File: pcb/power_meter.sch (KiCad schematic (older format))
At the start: 46 parts, among them J1 USB_B, J2 AudioJack3, J3 Conn_Coaxial, U1 LD1117S33TR_SOT223, U2 ATmega32U4-MU, U3 nRF24L01P, U4 RFX2401C, Y1 16 MHz, Y2 16 MHz

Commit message: separate schematic in multiple sheets; annotate components; power section
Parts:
- removed C? (x2): 22 pF, symbol Device:C
- removed C?: 10 nF, symbol Device:C
- removed C?: 1 nF, symbol Device:C
- removed C?: 33 nF, symbol Device:C
- removed C? (x5): 1.5 pF, symbol Device:C
- removed C?: 0.3 pF, symbol Device:C
- removed C?: 220 pF, symbol Device:C
- removed C?: 1 uF, symbol Device:C
- removed C?: 1 pF, symbol Device:C
- removed C?: 2.2 nF, symbol Device:C
- removed C?: 4.7 nF, symbol Device:C
- removed J3: Conn_Coaxial, symbol Connector:Conn_Coaxial
- removed L? (x2): 2.4 nH, symbol Device:L
- removed L?: 8.2 nH, symbol Device:L
- removed L?: 3.9 nH, symbol Device:L
- removed L?: 2.7 nH, symbol Device:L
- removed R?: 1M, symbol Device:R
- removed R?: 22k, symbol Device:R
- removed R? (x2): 1k, symbol Device:R
- removed R?: 20k, symbol Device:R
- removed U3: nRF24L01P, Package_DFN_QFN:QFN-20-1EP_4x4mm_P0.5mm_EP2.5x2.5mm, symbol RF:nRF24L01P
- removed U4: RFX2401C, QFN50P300X300X60-17N, symbol power_meter-rescue:RFX2401C-RFX2401C
- removed Y2: 16 MHz, symbol Device:Crystal
- added C1, C4: 1 uF, symbol Device:C
- added C2, C3: 10 uF, symbol Device:C
- added C5: 100 nF, symbol Device:C
- added D1: D, symbol Device:D
- added F1: Polyfuse, symbol Device:Polyfuse
- added LOGO1: Logo_Open_Hardware_Small, Symbol:OSHW-Logo2_9.8x8mm_SilkScreen, symbol Graphic:Logo_Open_Hardware_Small
- C10, C7, C8, C9: renamed from C?; footprint (none) -> Capacitor_SMD:C_0402_1005Metric
- J1: footprint (none) -> Connector_USB:USB_B_Lumberg_2411_02_Horizontal
- J2: footprint (none) -> Connector_Audio:Jack_3.5mm_CUI_SJ-3523-SMT_Horizontal
- R5: renamed from R?; footprint (none) -> Resistor_SMD:R_0402_1005Metric
- gave numbers to parts that had none: 4
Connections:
- net GND: now also U1.1 (GND), C1.2, C2.2, C3.2, C4.2, C5.2
- net VBUS: now also U2.14 (VCC), U2.24 (AVCC), U2.34 (VCC), U2.44 (AVCC), C1.1, F1.2
- net VCC: no longer U2.24 (AVCC), U2.44 (AVCC)
- net VDD: now also U1.2 (VO), C3.1, C4.1, C5.1
- net at U1.3 (VI): now also C2.1, D1.1 (K)
- net NRF_SCK renamed SCK
- new net: D1.2 (A), F1.1
- no-connect marks 23 -> 22
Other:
- note added: "Power"
- note added: "Shield is grounded at the\nhost side.\n22 Ohm resistors are\nrequired by the USB standard.\nUSB standard mandatas input\ncapacitance <= 10 uF."
- note added: "USB Connector & Decoupling"
- note removed: "Antenna Matching Network"
- note removed: "Conversion to Unbalanced & Impedance Matching Network"
- note removed: "Decoupling & Support Circuitry"
- note removed: "Nordic Semiconductors nRF24L01P"
- note removed: "RFAxis RFX2401C"
- note removed: "SMA Connector"
- note removed: "Shield is grounded at the\nhost side.\n22 Ohm resistors are\nrequired by the USB standard."
- note removed: "TODO: LINK TO ORIGINAL SCHEMATIC"
- note removed: "USB Connector"
- moved on the sheet: C6, D2, J1, J2, R1, R2, R3, R4, U1

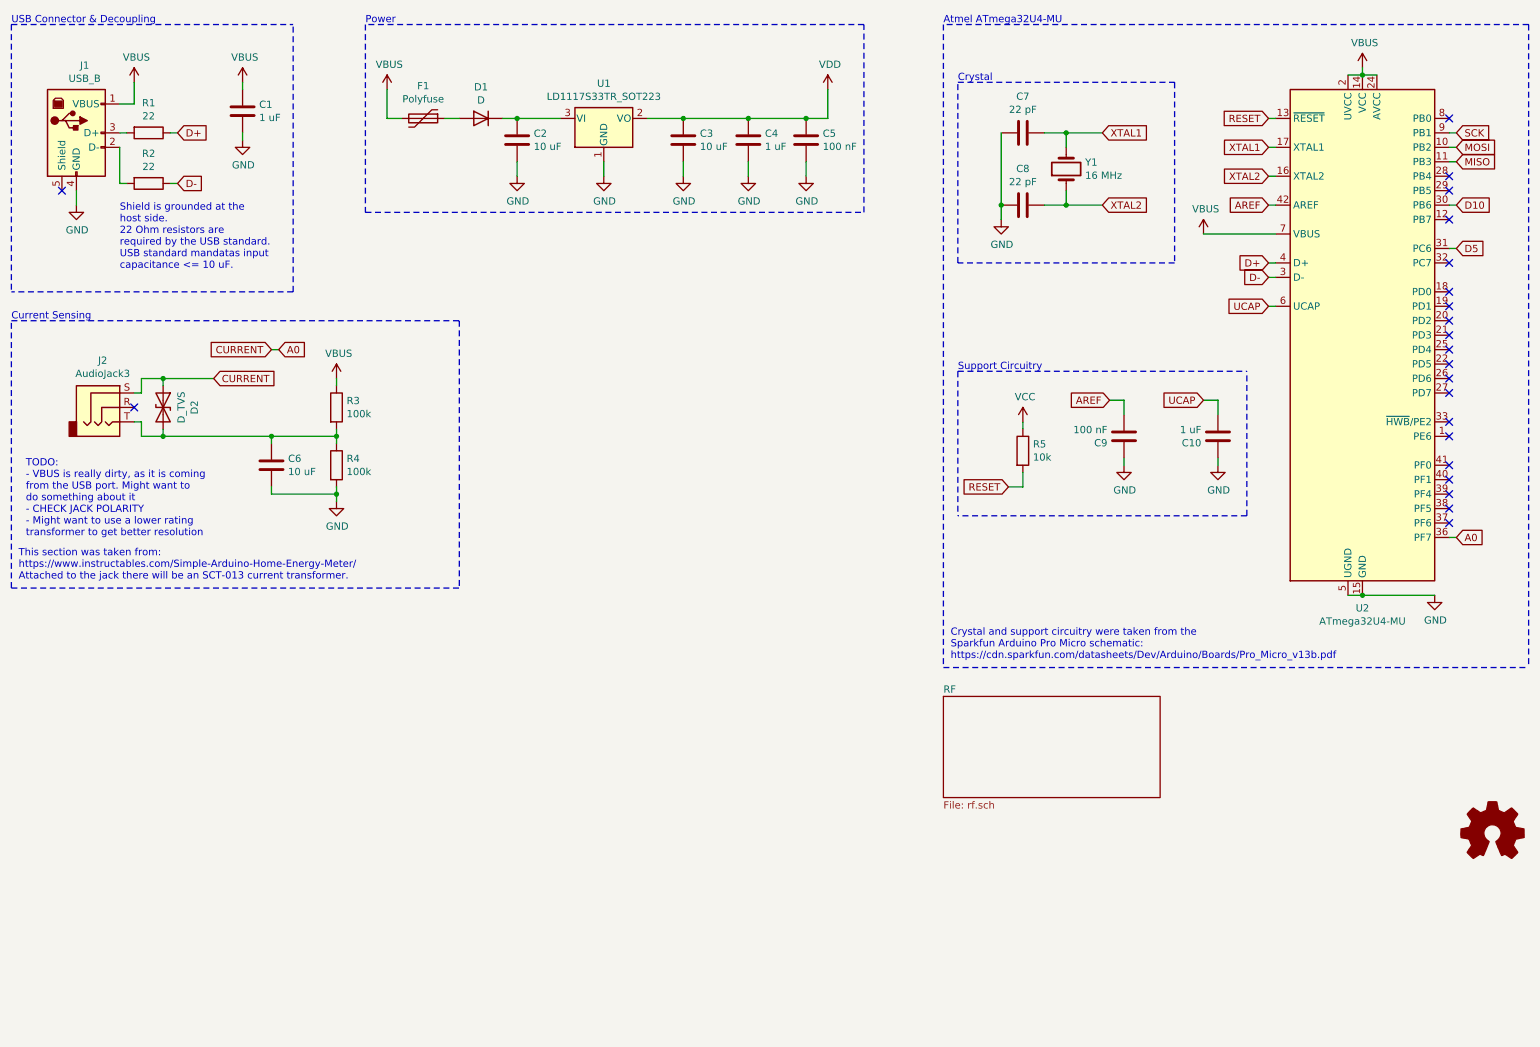
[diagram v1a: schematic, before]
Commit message: add more decoupling caps and notes
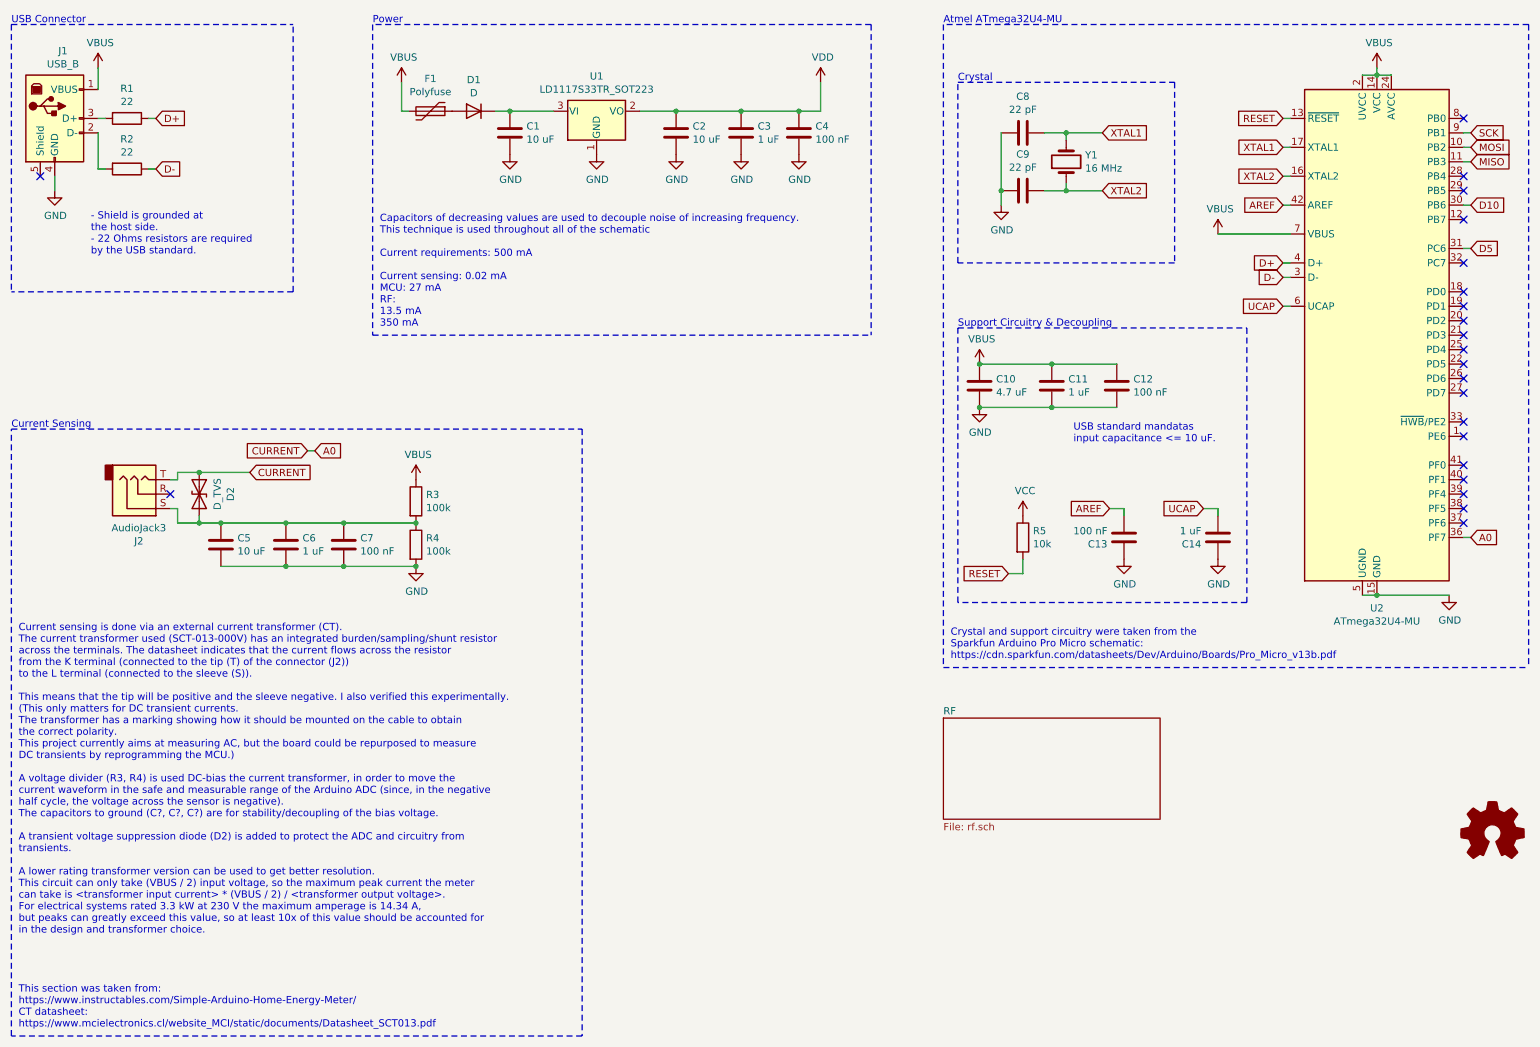
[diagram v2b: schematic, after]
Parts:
- added C11: 1 uF, symbol Device:C
- added C12, C7: 100 nF, symbol Device:C
- added C5: 10 uF, symbol Device:C
- C10: renamed from C1; value 1 uF -> 4.7 uF
- C6: value 10 uF -> 1 uF
- renumbered C2 to C1, C9 to C13, C10 to C14, C3 to C2, C4 to C3, C5 to C4, C7 to C8, C8 to C9
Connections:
- net A0: now also J2.T; no longer J2.S
- net GND: now also C11.2, C12.2, C5.2, C7.2
- net VBUS: now also C11.1, C12.1
- net at C6.1, D2.2 (A2), R3.2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: now also J2.S, C5.1, C7.1; no longer J2.T
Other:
- note added: "- Shield is grounded at\nthe host side.\n- 22 Ohms resistors are required\nby the USB standard."
- note added: "Capacitors of decreasing values are used to decouple noise of increasing frequency.\nThis technique is used throughout all of the schematic\n\nCurrent requirements: 500 mA\n\nCurrent sensing: 0.02 mA\nMCU: 27 mA\nRF:\n13.5 mA\n350 mA"
- note added: "Current sensing is done via an external current transformer (CT).\nThe current transformer used (SCT-013-000V) has an integrated burden/sampling/shunt resistor\nacross the terminals. The datasheet indicates that the current flows across the resistor\nfrom the K terminal (connected to the tip (T) of the connector (J2))\nto the L terminal (connected to the sleeve (S)).\n\nThis means that the tip wi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"
- note added: "Support Circuitry & Decoupling"
- note added: "This section was taken from:\nhttps://www.instructables.com/Simple-Arduino-Home-Energy-Meter/\nCT datasheet:\nhttps://www.mcielectronics.cl/website_MCI/static/documents/Datasheet_SCT013.pdf"
- note added: "USB Connector"
- note added: "USB standard mandatas\ninput capacitance <= 10 uF."
- note removed: "Shield is grounded at the\nhost side.\n22 Ohm resistors are\nrequired by the USB standard.\nUSB standard mandatas input\ncapacitance <= 10 uF."
- note removed: "Support Circuitry"
- note removed: "TODO:\n- VBUS is really dirty, as it is coming\nfrom the USB port. Might want to\ndo something about it\n- CHECK JACK POLARITY\n- Might want to use a lower rating\ntransformer to get better resolution"
- note removed: "This section was taken from:\nhttps://www.instructables.com/Simple-Arduino-Home-Energy-Meter/\nAttached to the jack there will be an SCT-013 current transformer."
- note removed: "USB Connector & Decoupling"
- moved on the sheet: C1, C10, C13, C14, C2, C3, C4, C6, C9, D1, D2, F1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
